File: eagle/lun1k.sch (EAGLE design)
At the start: 101 parts, among them IC1 LTC3558, IC2 LM27313, IC3 STM32F405RGT, IC4 NRF24L01SMD, J2 XF2-3015-1LW, Q1 Q12M-SMD-S, Q2 3.2X2.5CRYSTAL, SW1 JS102011SAQN, SW2 SWITCH_MCTAEF, SW3 SWITCH_MCTAEF, SW4 SWITCH_MCTAEF, U1 N35P112, X1 MICROUSB, X1_ JST-PH3

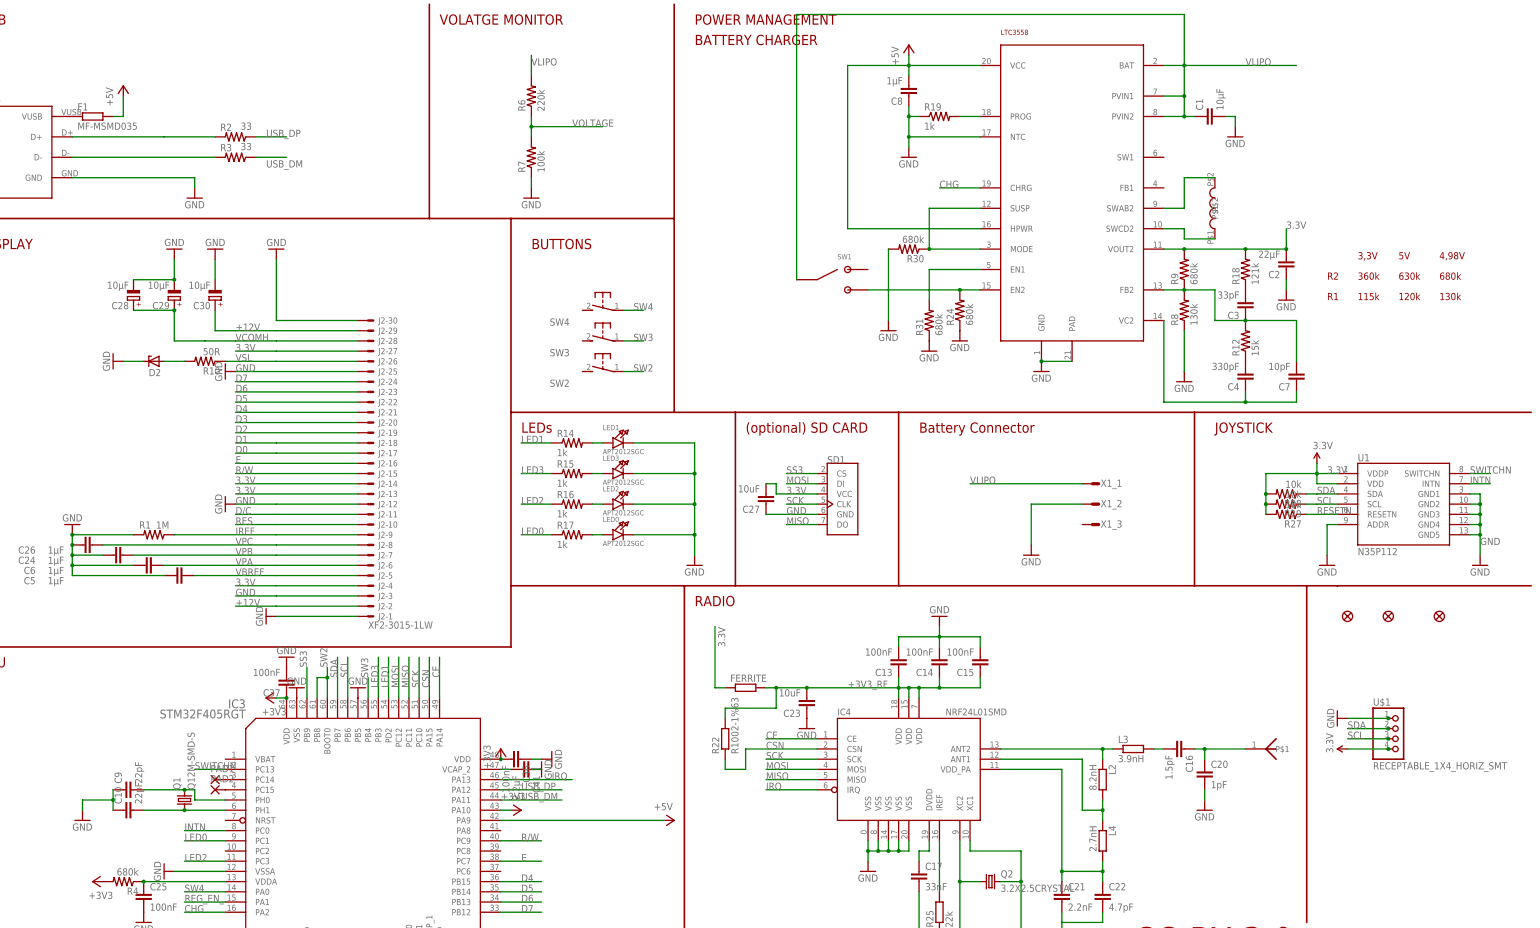
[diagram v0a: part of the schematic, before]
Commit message: routing
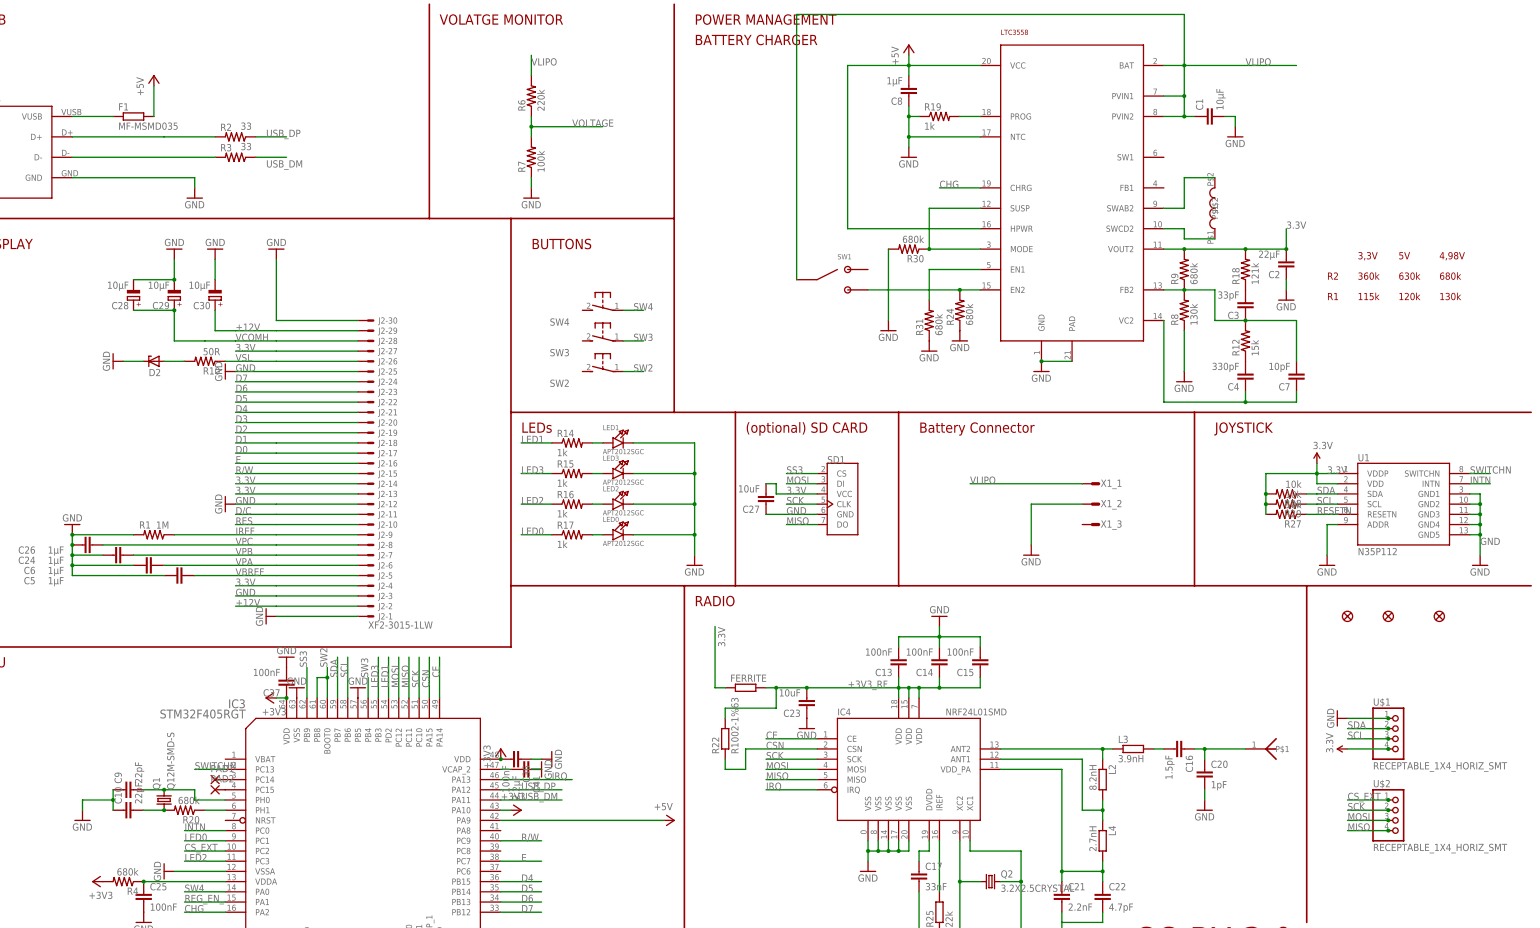
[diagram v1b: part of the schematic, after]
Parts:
- added R20: 680k, SparkFun-Resistors:RESISTOR0402-RES
- added U$2: RECEPTABLE_1X4_HORIZ_SMT, seb:RECEPTABLE_1X4_HORIZ_SMT
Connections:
- new net CS_EXT: IC3.PC2, U$2.1, U$2.1@1
- new net N$28: IC3.PH1, R20.1
- net MISO: now also U$2.4, U$2.4@1
- net MOSI: now also U$2.3, U$2.3@1
- net N$3: now also R20.2; no longer IC3.PH1
- net SCK: now also U$2.2, U$2.2@1
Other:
- moved on the sheet: F1, Q1
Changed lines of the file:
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@@
 <part name="C33" library="SparkFun" deviceset="CAP" device="0805" value="1µF"/>
 <part name="R11" library="rcl" deviceset="R-EU_" device="R0402" value="15k"/>
+<part name="R20" library="SparkFun-Resistors" deviceset="RESISTOR" device="0402-RES" value="680k"/>
+<part name="U$2" library="seb" deviceset="RECEPTABLE_1X4_HORIZ_SMT" device=""/>
 </parts>
 <sheets>
@@
 <wire x1="231.14" y1="119.38" x2="231.14" y2="162.56" width="0.4064" layer="94"/>
 <wire x1="231.14" y1="119.38" x2="304.8" y2="119.38" width="0.4064" layer="94"/>
-<wire x1="304.8" y1="119.38" x2="340.36" y2="119.38" width="0.4064" layer="94"/>
-<wire x1="340.36" y1="119.38" x2="388.62" y2="119.38" width="0.4064" layer="94"/>
+<wire x1="304.8" y1="119.38" x2="388.62" y2="119.38" width="0.4064" layer="94"/>
 <wire x1="177.8" y1="119.38" x2="177.8" y2="0" width="0.4064" layer="94"/>
 <wire x1="332.74" y1="119.38" x2="332.74" y2="35.56" width="0.4064" layer="94"/>
@@
 <instance part="R14" gate="G$1" x="149.86" y="154.94"/>
 <instance part="C9" gate="G$1" x="40.64" y="68.58" rot="R90"/>
-<instance part="P+5" gate="1" x="38.1" y="243.84"/>
+<instance part="P+5" gate="1" x="45.72" y="246.38"/>
 <instance part="GND9" gate="1" x="55.88" y="215.9"/>
 <instance part="R2" gate="G$1" x="66.04" y="231.14" smashed="yes" rot="R180">
@@
 </instance>
 <instance part="GND11" gate="1" x="180.34" y="124.46"/>
-<instance part="Q1" gate="G$1" x="53.34" y="66.04" rot="R90"/>
+<instance part="Q1" gate="G$1" x="48.26" y="66.04" rot="R90"/>
 <instance part="C10" gate="G$1" x="40.64" y="63.5" rot="R90"/>
 <instance part="GND13" gate="1" x="27.94" y="60.96"/>
@@
 <instance part="FRAME1" gate="G$1" x="0" y="0"/>
 <instance part="FRAME1" gate="G$2" x="287.02" y="0"/>
-<instance part="F1" gate="G$1" x="30.48" y="236.22"/>
+<instance part="F1" gate="G$1" x="40.64" y="236.22"/>
 <instance part="SD1" gate="SD" x="213.36" y="139.7"/>
 <instance part="IC4" gate="G$1" x="233.68" y="73.66"/>
@@
 <instance part="C33" gate="G$1" x="154.94" y="-43.18"/>
 <instance part="R11" gate="G$1" x="187.96" y="-43.18" rot="R90"/>
+<instance part="R20" gate="G$1" x="53.34" y="63.5" rot="R180"/>
+<instance part="U$2" gate="G$1" x="353.06" y="60.96"/>
 </instances>
 <busses>
@@
 <pinref part="F1" gate="G$1" pin="2"/>
 <pinref part="P+5" gate="1" pin="+5V"/>
-<wire x1="35.56" y1="236.22" x2="38.1" y2="236.22" width="0.1524" layer="91"/>
-<wire x1="38.1" y1="236.22" x2="38.1" y2="241.3" width="0.1524" layer="91"/>
+<wire x1="45.72" y1="236.22" x2="45.72" y2="243.84" width="0.1524" layer="91"/>
 </segment>
 <segment>
@@
 <net name="N$1" class="0">
 <segment>
-<wire x1="53.34" y1="68.58" x2="55.88" y2="68.58" width="0.1524" layer="91"/>
+<wire x1="48.26" y1="68.58" x2="55.88" y2="68.58" width="0.1524" layer="91"/>
 <wire x1="55.88" y1="68.58" x2="55.88" y2="66.04" width="0.1524" layer="91"/>
 <wire x1="55.88" y1="66.04" x2="63.5" y2="66.04" width="0.1524" layer="91"/>
-<wire x1="43.18" y1="68.58" x2="53.34" y2="68.58" width="0.1524" layer="91"/>
-<junction x="53.34" y="68.58"/>
+<wire x1="43.18" y1="68.58" x2="48.26" y2="68.58" width="0.1524" layer="91"/>
+<junction x="48.26" y="68.58"/>
 <pinref part="Q1" gate="G$1" pin="2"/>
 <pinref part="C9" gate="G$1" pin="2"/>
@@
 <net name="N$3" class="0">
 <segment>
-<wire x1="63.5" y1="63.5" x2="53.34" y2="63.5" width="0.1524" layer="91"/>
-<wire x1="43.18" y1="63.5" x2="53.34" y2="63.5" width="0.1524" layer="91"/>
-<junction x="53.34" y="63.5"/>
+<wire x1="43.18" y1="63.5" x2="48.26" y2="63.5" width="0.1524" layer="91"/>
 <pinref part="Q1" gate="G$1" pin="1"/>
 <pinref part="C10" gate="G$1" pin="2"/>
-<pinref part="IC3" gate="G$1" pin="PH1"/>
+<pinref part="R20" gate="G$1" pin="2"/>
+<junction x="48.26" y="63.5"/>
 </segment>
 </net>
@@
 <pinref part="IC3" gate="G$1" pin="PC11"/>
 </segment>
+<segment>
+<pinref part="U$2" gate="G$1" pin="4"/>
+<wire x1="353.06" y1="58.42" x2="342.9" y2="58.42" width="0.1524" layer="91"/>
+<label x="342.9" y="58.42" size="1.778" layer="95"/>
+<pinref part="U$2" gate="G$1" pin="4@1"/>
+<junction x="353.06" y="58.42"/>
+</segment>
 </net>
 <net name="MOSI" class="0">
@@
 <pinref part="IC3" gate="G$1" pin="PC12"/>
 </segment>
+<segment>
+<pinref part="U$2" gate="G$1" pin="3"/>
+<wire x1="353.06" y1="60.96" x2="342.9" y2="60.96" width="0.1524" layer="91"/>
+<label x="342.9" y="60.96" size="1.778" layer="95"/>
+<pinref part="U$2" gate="G$1" pin="3@1"/>
+<junction x="353.06" y="60.96"/>
+</segment>
 </net>
 <net name="SCK" class="0">
@@
 <label x="111.76" y="93.98" size="1.778" layer="95" rot="R90"/>
 <pinref part="IC3" gate="G$1" pin="PC10"/>
+</segment>
+<segment>
+<pinref part="U$2" gate="G$1" pin="2"/>
+<wire x1="353.06" y1="63.5" x2="342.9" y2="63.5" width="0.1524" layer="91"/>
+<label x="342.9" y="63.5" size="1.778" layer="95"/>
+<pinref part="U$2" gate="G$1" pin="2@1"/>
+<junction x="353.06" y="63.5"/>
 </segment>
 </net>
@@
 <pinref part="X1" gate="G$1" pin="VUSB"/>
 <pinref part="F1" gate="G$1" pin="1"/>
+<wire x1="35.56" y1="236.22" x2="25.4" y2="236.22" width="0.1524" layer="91"/>
 </segment>
 </net>
@@
 </segment>
 </net>
+<net name="N$28" class="0">
+<segment>
+<pinref part="R20" gate="G$1" pin="1"/>
+<pinref part="IC3" gate="G$1" pin="PH1"/>
+<wire x1="58.42" y1="63.5" x2="63.5" y2="63.5" width="0.1524" layer="91"/>
+</segment>
+</net>
+<net name="CS_EXT" class="0">
+<segment>
+<pinref part="U$2" gate="G$1" pin="1"/>
+<wire x1="353.06" y1="66.04" x2="342.9" y2="66.04" width="0.1524" layer="91"/>
+<label x="342.9" y="66.04" size="1.778" layer="95"/>
+<pinref part="U$2" gate="G$1" pin="1@1"/>
+<junction x="353.06" y="66.04"/>
+</segment>
+<segment>
+<pinref part="IC3" gate="G$1" pin="PC2"/>
+<wire x1="63.5" y1="53.34" x2="53.34" y2="53.34" width="0.1524" layer="91"/>
+<label x="53.34" y="53.34" size="1.778" layer="95"/>
+</segment>
+</net>
